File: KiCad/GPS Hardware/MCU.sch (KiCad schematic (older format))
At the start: 16 parts, among them J2 Conn_01x06_Male, U5 ATmega328-AU, U6 SN74AVC4T774PW, Y1 Crystal

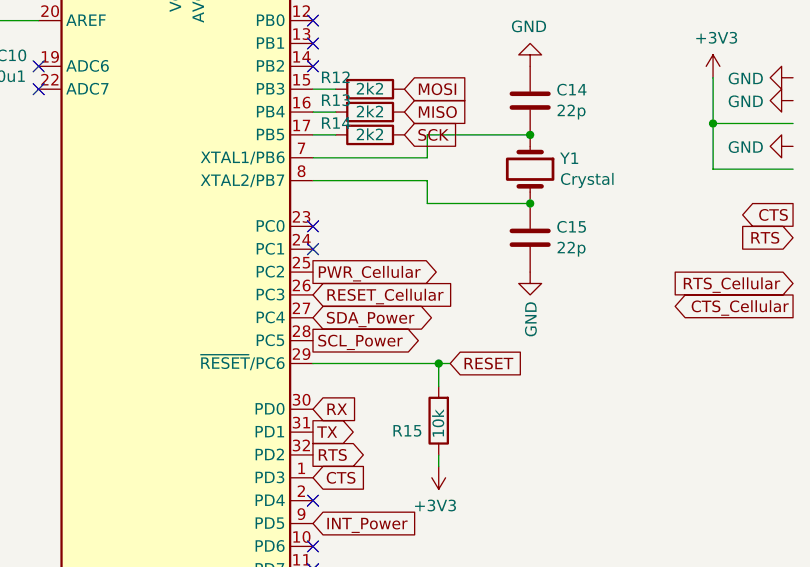
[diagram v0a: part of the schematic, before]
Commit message: Update to PC
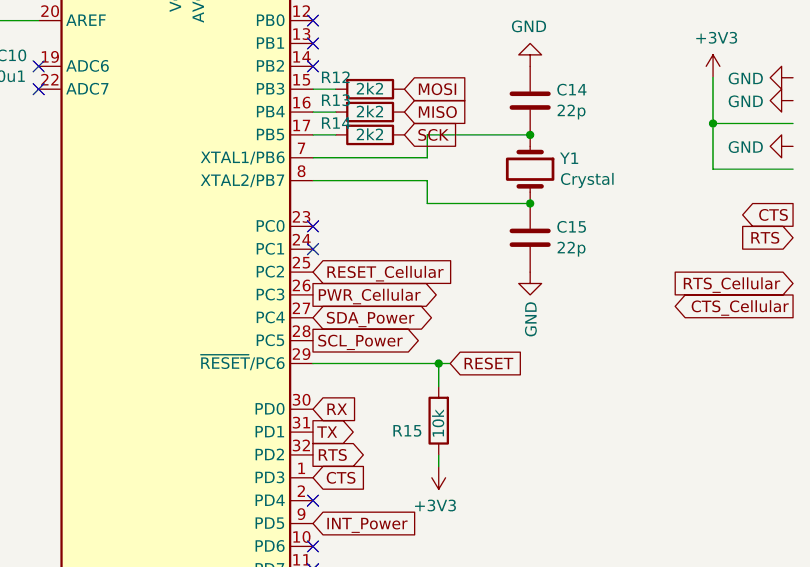
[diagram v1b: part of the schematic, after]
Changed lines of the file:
@@
 	1    0    0    -1
 $EndComp
-Text GLabel 3450 3100 2    50   Output ~ 0
+Text GLabel 3450 3200 2    50   Output ~ 0
 PWR_Cellular
-Text GLabel 3450 3200 2    50   Input ~ 0
+Text GLabel 3450 3100 2    50   Input ~ 0
 RESET_Cellular
 NoConn ~ 2250 2200
